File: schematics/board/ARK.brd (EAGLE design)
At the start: 89 x 89 mm, 82 parts, among them IC2 STM32F103C8T, Q5 8MHz

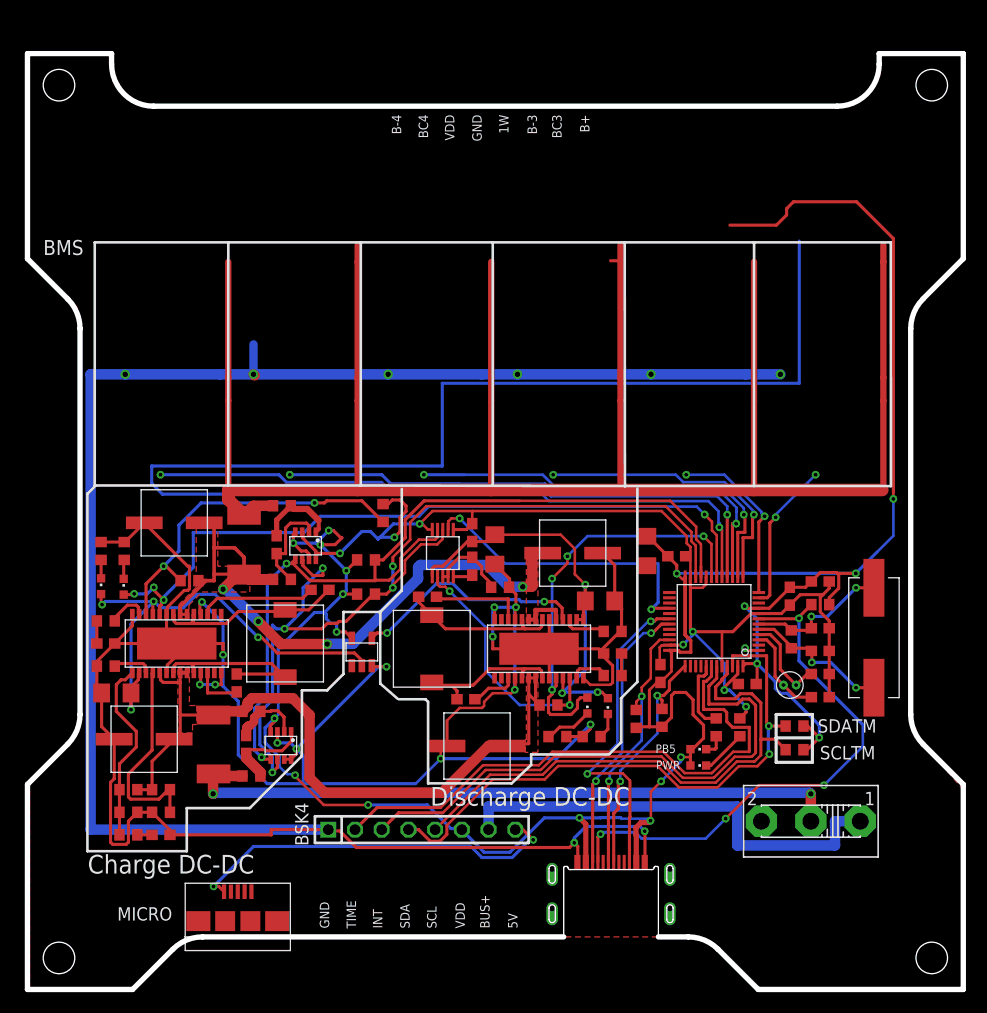
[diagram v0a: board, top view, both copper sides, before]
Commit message: Добавлены герберы плат BSK1-4, PL, SP и SPIDER
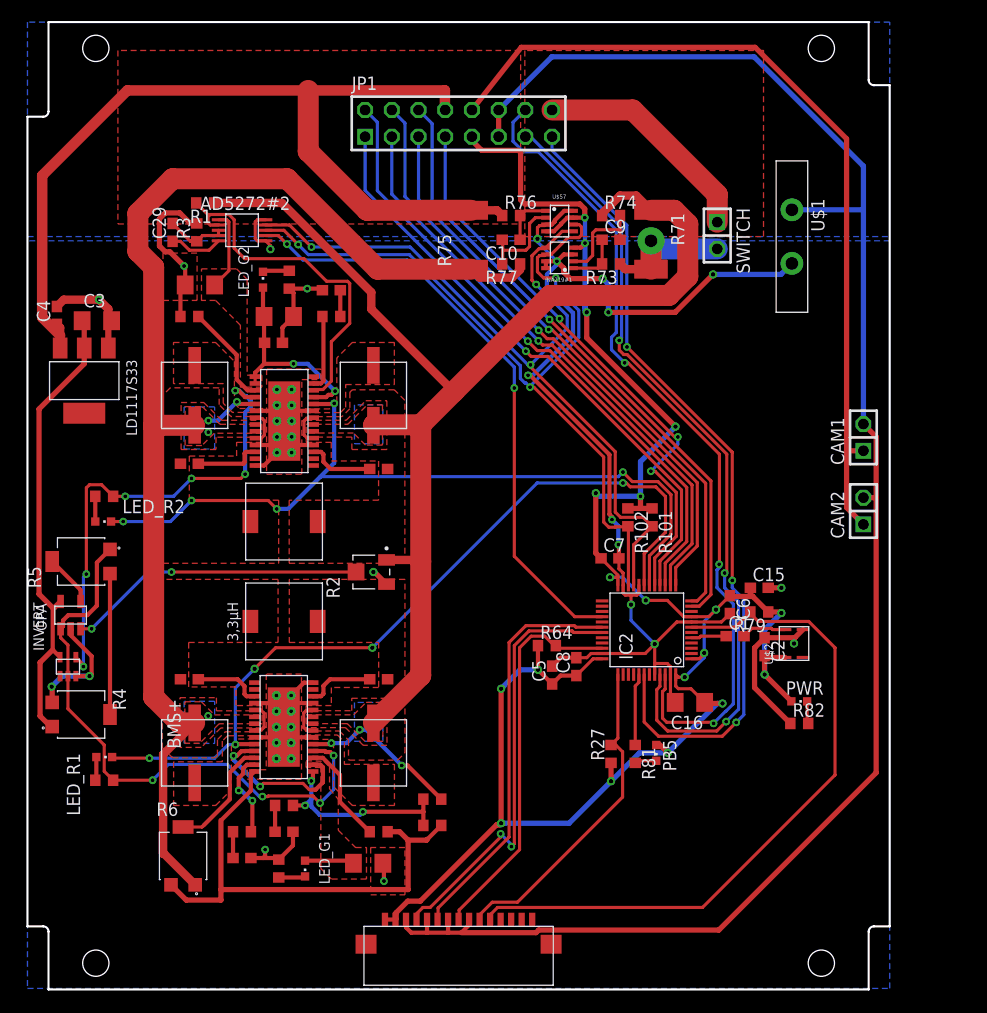
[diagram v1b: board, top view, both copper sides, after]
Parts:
- removed BSK4: (no value), pinheadCS:1X08
- removed C005R: 32,768KHz, CanCubeSat:C005R
- removed C13, C14, C33, C34, C51: 0,1µ, rcl:C0603
- removed C30, C36: 680p, rcl:C0603
- removed C31, C39: 4.7µ, rcl:C1206
- removed C35: 150µ, CanCubeSat:ECAP150
- removed C37: 220µ, CanCubeSat:ECAP220
- removed C38: 3,3n, rcl:C0603
- removed LED1, LED2, LED3, LED8: (no value), led:CHIPLED_0603
- removed MICRO: 629105136821, MicroUSB:629105136821
- removed Q5: 8MHz, 9C-8.000MEEJ-T:XTAL_9C-8.000MEEJ-T
- removed R25, R26: 5k1, resistor:R0603
- removed R29: 150k, resistor:R0603
- removed R31: 2k, resistor:R0603
- removed R61: 91K, resistor:R0603
- removed R62, R72: 232k, resistor:R0603
- removed R70: 24k3, resistor:R0603
- removed R78: 1M, resistor:R0603
- removed R87: 680k, resistor:R0603
- removed S1: (no value), cansat-lib:UNICS-SWITCH
- removed U$16: LTC3119, CanCubeSat:LTC3119
- added C1: 1nF, rcl:C0603
- added C10, C56, C9: 0,1µ, rcl:C0603
- added C2: 10nF, rcl:C0603
- added C3, C57: 10µ, rcl:C1206
- added C4, C5, C6, C7, C8: 100nF, rcl:C0603
- added CAM1, CAM2, SWITCH: (no value), pinheadCS:1X02
- added INVERT: INVERTER., CanCubeSat:SC70
- added JP1: (no value), pinheadCS:2X08
- added LD1117S33: LD1117S33, CanCubeSat:SOT223
- added LED_G1, LED_G2, LED_R1, LED_R2: (no value), led:CHIPLED_0603
- added OPA: OPA333, CanCubeSat:SOT23-5
- added R1: 91K, resistor:R0603
- added R2: 3313J-1-205E, CanCubeSat:TRIM_3313J-1-205E
- added R3: 14K3, resistor:R0603
- added R33: 2k, resistor:R0603
- added R4, R5, R6: 3314G-1-504E, CanCubeSat:TRIM_3314G-1-504E
- added U$1: MF-R400, CanCubeSat:MF-R400
- added U$12: FFC-CONNECT68611, CanCubeSat:68611
- 3,3µH1: value 3,3µ -> 3,3µH
- AD5272#2: device CanCubeSat:AD5272 -> CanCubeSat:MSOP10
- C44: value 27pF -> 680p
- C45: value 27pF -> 4.7µ; device rcl:C0603 -> rcl:C1206
- C46: value 10pF -> 3,3n
- C47: value 10pF -> 150µ; device rcl:C0603 -> CanCubeSat:ECAP150-CMD
- C48, C55: value 100nF -> 220µ; device rcl:C0603 -> CanCubeSat:ECAP220-CMD
- C49: value 150µ -> 0,1µ; device CanCubeSat:ECAP150 -> rcl:C0603
- C50: value 220µ -> 0,1µ; device CanCubeSat:ECAP220 -> rcl:C0603
- C52: value 10µ -> 680p; device rcl:C1206 -> rcl:C0603
- C53: value 100nF -> 4.7µ; device rcl:C0603 -> rcl:C1206
- C54: value 100nF -> 150µ; device rcl:C0603 -> CanCubeSat:ECAP150-CMD
- INA219#1, U$57: device CanCubeSat:INA219AID -> CanCubeSat:SOT23-8
- R30: value 14K3 -> 150k
- U$2: value INVERTER -> Q24; device CanCubeSat:INVERTER -> CanCubeSat:Q24
- U$23: value USB-C -> LTC31191; device CanCubeSat:USB-C -> CanCubeSat:LTC3119+VIA
- U$59: value LTC3119 -> LTC31191; device CanCubeSat:LTC3119 -> CanCubeSat:LTC3119+VIA
- moved C53 64.4 mm to (16.4, 67.0)
- moved R71 63.5 mm to (59.3, 71.3)
- moved C47 60.0 mm to (15.9, 22.5)
- moved R73 59.5 mm to (55.5, 69.0), turned to 180 degrees
- moved C44 59.2 mm to (20.4, 12.5)
- moved R74 58.2 mm to (55.5, 73.6)
- moved U$23 58.1 mm to (24.4, 54.1), turned to 90 degrees
- moved INA219#1 53.4 mm to (50.6, 69.6), turned to 180 degrees
- moved C46 52.6 mm to (24.4, 15.0)
- moved C55 51.6 mm to (15.9, 56.5), turned to 180 degrees
- moved R28 50.2 mm to (15.4, 64.0), turned to 0 degrees
- moved R57 48.8 mm to (7.30, 46.9)
- moved C45 47.5 mm to (32.4, 12.0)
- moved C48 45.5 mm to (32.9, 22.5)
- moved C54 44.0 mm to (32.9, 56.5), turned to 180 degrees
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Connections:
- removed net I2CINT: BSK4.3, IC2.43
- removed net N$11: 3,3µH1.2, C13.1, U$16.21, U$16.24
- removed net N$12: 3,3µH1.1, C14.1, U$16.5, U$16.8
- removed net N$133: C44.1, IC2.6, Q5.1, R78.1
- removed net N$145: C45.1, IC2.5, Q5.2, R78.2
- removed net N$148: C005R.P$2, C47.1, IC2.4
- removed net N$152: C005R.P$1, C46.1, IC2.3
- removed net N$25: R70.1, R72.1, U$59.12
- removed net N$26: LED1.C, R31.2
- removed net N$29: R28.2, U$16.17
- removed net N$32: C13.2, U$16.26
- removed net N$41: R29.1, U$16.13
- removed net N$42: C30.1, R29.2
- removed net N$47: AD5272#2.1, C31.1, C51.1, C52.1, LED1.A, U$16.11, U$16.15, U$16.16
- removed net N$5: AD5272#2.2, R61.1, U$16.12
- removed net N$52: C14.2, U$16.3
- removed net N$54: LED2.C, R32.2
- removed net N$55: R62.2, R87.1, U$59.18
- removed net N$56: LED3.C, R57.2
- removed net N$60: LED8.C, R100.2
- removed net RX-C: IC2.31, U$23.RX0
- removed net TX-C: IC2.30, U$23.TX0
- removed net VDD: BSK4.6, C15.1, C16.1, C48.1, C53.1, C54.1, C55.1, IC2.1, IC2.24, IC2.36, IC2.48, IC2.9, INA219#1.4, PB5.A, PWR.A, R101.1, R102.1, R25.1, R26.1, R27.1, R64.1, R79.1, U$2.P$5, U$23.3V3/BUS0, U$23.3V3/BUS1, U$57.4, U$57.7
- new net 1.65: R4.2, R5.3
- new net 302: OPA.P$4, R5.2
- new net 3V3: C15.1, C16.1, C2.2, C5.1, C6.1, C7.1, C8.1, IC2.1, IC2.24, IC2.36, IC2.48, IC2.9, INA219#1.4, JP1.9, PB5.A, PWR.A, R101.1, R102.1, R27.1, R64.1, R79.1, U$12.P$1, U$12.P$2, U$2.P$4, U$57.4, U$57.7
- new net 3V3-STAB: C3.1, INVERT.P$5, LD1117S33.P$3, OPA.P$5, R4.1
- new net GND-OUT: CAM1.2, CAM2.2, JP1.11, JP1.12, U$1.P$2, U$12.P$3, U$12.P$5, U$12.P$7, U$12.P$9
- new net N$1: C1.1, IC2.5
- new net N$215: AD5272#2.1, C53.1, C56.1, C57.1, LED_G2.A, U$23.11, U$23.15, U$23.16
- new net N$234: C45.1, LED_G1.A, U$59.11, U$59.16
- new net N$3: AD5272#2.2, R1.2, U$23.12
- new net N$4: C1.2, U$2.P$3
- new net N$77: 3,3µH1.2, C49.1, U$23.21, U$23.24
- new net N$78: 3,3µH1.1, C50.1, U$23.5, U$23.8
- new net N$79: R28.2, U$23.17
- new net N$80: C49.2, U$23.26
- new net N$81: R30.1, U$23.13
- new net N$82: C52.1, R30.2
- new net N$84: C50.2, U$23.3
- new net N$85: LED_R1.A, R32.2
- new net N$87: LED_R2.A, R57.2
- new net N$89: R6.2, U$59.12
- new net N$91: LED_G1.C, R100.2
- new net N$92: LED_G2.C, R33.2
- new net RUN: OPA.P$3, R2.2
- new net RX-S: IC2.31, U$12.P$4
- new net TX-S: IC2.30, U$12.P$6
- net 1W: now also JP1.7
- net 5V: now also CAM1.1, CAM2.1, JP1.10; no longer BSK4.8, MICRO.5V
- net A: now also INVERT.P$2, OPA.P$1, R32.1, R5.1, U$59.18; no longer C39.1, LED8.A, U$2.P$2, U$59.11, U$59.16
- net BMS+: now also C4.1, JP1.8, LD1117S33.P$4
- net BMS1: now also IC2.16, JP1.1; no longer IC2.15
- net BMS2: now also IC2.15, JP1.2; no longer IC2.16
- net BMS3: now also IC2.14, JP1.3; no longer IC2.13
- net BMS4: now also IC2.13, JP1.4; no longer IC2.14
- net BMS5: now also IC2.12, JP1.5; no longer IC2.11
- net BMS6: now also IC2.11, JP1.6; no longer IC2.12
- net BUS+: now also SWITCH.2; no longer S1.2
- net BUSPLUS: now also JP1.16, SWITCH.1; no longer BSK4.7, S1.1
- net GND: now also C2.1, C3.2, C4.2, C47.P$2, C48.P$2, C5.2, C54.P$2, C55.P$2, C56.2, C57.2, C6.2, C7.2, C8.2, INVERT.P$3, LD1117S33.P$2, OPA.P$2, R2.3, R3.2, R33.1, R4.3, R6.3, U$1.P$1, U$2.P$2, U$23.14, U$23.20, U$23.25, U$23.28, U$23.29, U$23.4, U$23.9, U$23.P$1, U$23.P$10, U$23.P$2, U$23.P$3, U$23.P$4, U$23.P$5, U$23.P$6, U$23.P$7, U$23.P$8, U$23.P$9, U$59.P$1, U$59.P$10, U$59.P$2, U$59.P$3, U$59.P$4, U$59.P$5, U$59.P$6, U$59.P$7, U$59.P$8, U$59.P$9; no longer BSK4.1, C30.2, C31.2, C35.P$2, C36.2, C37.P$2, C38.2, C39.2, C47.2, C48.2, C49.P$2, C50.P$2, C51.2, C54.2, C55.2, MICRO.GND, MICRO.Z1, MICRO.Z2, MICRO.Z3, MICRO.Z4, R30.2, R31.1, R32.1, R57.1, R62.1, R70.2, U$16.14, U$16.20, U$16.25, U$16.28, U$16.29, U$16.4, U$16.9, U$2.P$3, U$23.GND0, U$23.GND1
- net INA_BMS+: now also C47.P$1, C55.P$1, R6.1, U$23.19, U$23.22, U$23.23; no longer C35.P$1, C50.P$1, R72.2, U$16.19, U$16.22, U$16.23
- net INA_BUS+: now also C48.P$1, C54.P$1, R1.1, R2.1, U$23.6, U$23.7; no longer C37.P$1, C49.P$1, R61.2, R87.2, U$16.6, U$16.7
- net N$129: now also C41.2; no longer C34.2
- net N$131: now also C40.1; no longer C33.1
- net N$132: now also C41.1; no longer C34.1
- net N$136: now also C44.1; no longer C36.1
- net N$139: now also C46.1; no longer C38.1
- net N$14: now also C9.2; no longer C40.2
- net N$144: now also C40.2; no longer C33.2
- net N$147: now also C9.1; no longer C40.1
- net N$150: now also C10.1; no longer C41.1
- net N$151: now also C10.2; no longer C41.2
- net N$48: now also R3.1; no longer R30.1
- net NRST: now also U$12.P$11; no longer U$23.NRST/EN
- net PGOOD1: now also IC2.19, LED_R1.C; no longer IC2.18, LED2.A
- net PGOOD2: now also IC2.18, LED_R2.C, U$23.10; no longer IC2.19, LED3.A, U$16.10
- net SCLTM: now also JP1.13; no longer BSK4.5, R25.2
- net SDATM: now also JP1.14; no longer BSK4.4, R26.2
- net SWC: now also U$12.P$10; no longer U$23.SWC/TXD
- net SWD: now also U$12.P$8; no longer U$23.SWD/RXD
- net TIME: now also JP1.15; no longer BSK4.2
- net Y: now also INVERT.P$4, R57.1, U$23.18; no longer U$16.18, U$2.P$4
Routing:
- net VDD: track 259.4 -> 0.00 mm, vias 20 -> 0
- net GND: track 520.3 -> 261.9 mm, vias 28 -> 21
- net 3V3: track 0.00 -> 194.2 mm, vias 0 -> 19
- net GND-OUT: track 0.00 -> 165.9 mm
- net BMS+: track 204.3 -> 88.6 mm
- net 1W: track 146.0 -> 55.1 mm, vias 1 -> 3
- net INA_BUS+: track 71.9 -> 131.1 mm, vias 0 -> 3
- net I2CINT: track 53.6 -> 0.00 mm
- net BUS+: track 64.3 -> 12.5 mm, vias 2 -> 1
- net INA_BMS+: track 74.2 -> 121.2 mm
- net 5V: track 36.4 -> 81.1 mm, vias 2 -> 0
- net 3V3-STAB: track 0.00 -> 44.1 mm
- net BMS6: track 16.6 -> 59.9 mm, vias 2 -> 1
- net BMS5: track 14.4 -> 56.5 mm, vias 2 -> 1
- net RX-S: track 0.00 -> 41.7 mm, vias 0 -> 2
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- added copper zone on layer 1, net BMS+
- added copper zone on layer 1, net BUSPLUS
- added copper zone on layer 16, net GND
- added copper zone on layer 16, net GND-OUT
- added copper zone on layer 16, net INA_BMS+
- added copper zone on layer 16, net INA_BUS+
- added copper zone on layer 1, net N$131
- added copper zone on layer 1, net N$132
- added copper zone on layer 1, net N$215
- added copper zone on layer 1, net N$234
- added copper zone on layer 1, net N$77
- added copper zone on layer 1, net N$78
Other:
- board size 89 x 89 mm -> 82 x 92 mm
- board text added: "BMS+"
- board text added: "LTC3119"
- board text removed: "1W"
- board text removed: "5V"
- board text removed: "ARK "Концерн ИТС""
- board text removed: "B+"
- board text removed: "B-3"
- board text removed: "B-4"
- board text removed: "BC3"
- board text removed: "BC4"
- board text removed: "BMS"
- board text removed: "BUS+"
- board text removed: "Charge DC-DC"
- board text removed: "Discharge DC-DC"
- board text removed: "GND"
- board text removed: "INT"
- board text removed: "OFF"
- board text removed: "ON"
- board text removed: "SCL"
- board text removed: "SCLTM"
- board text removed: "SDA"
- board text removed: "SDATM"
- board text removed: "TIME"
- board text removed: "VDD"
